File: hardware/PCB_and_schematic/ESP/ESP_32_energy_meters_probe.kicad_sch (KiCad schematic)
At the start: 31 parts, among them J2 Conn_01x10, J5 METER_GRID, J9 METER_PV, U4 ST485EBDR, U5 ST485EBDR, U6 74HC14

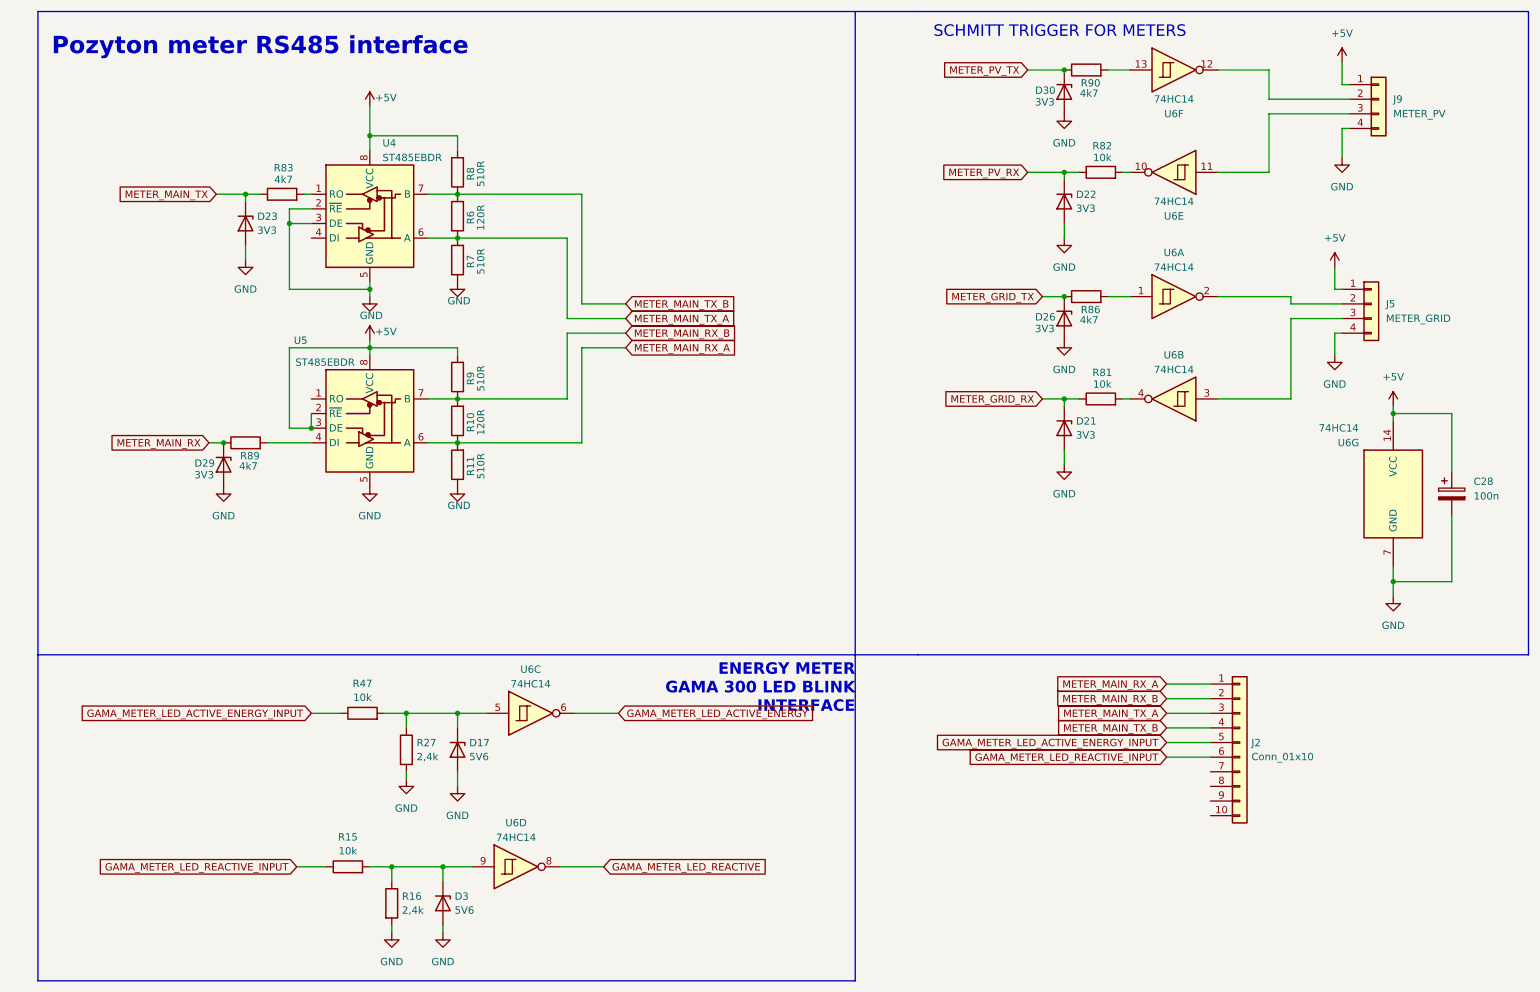
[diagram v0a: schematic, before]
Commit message: Routing PCB
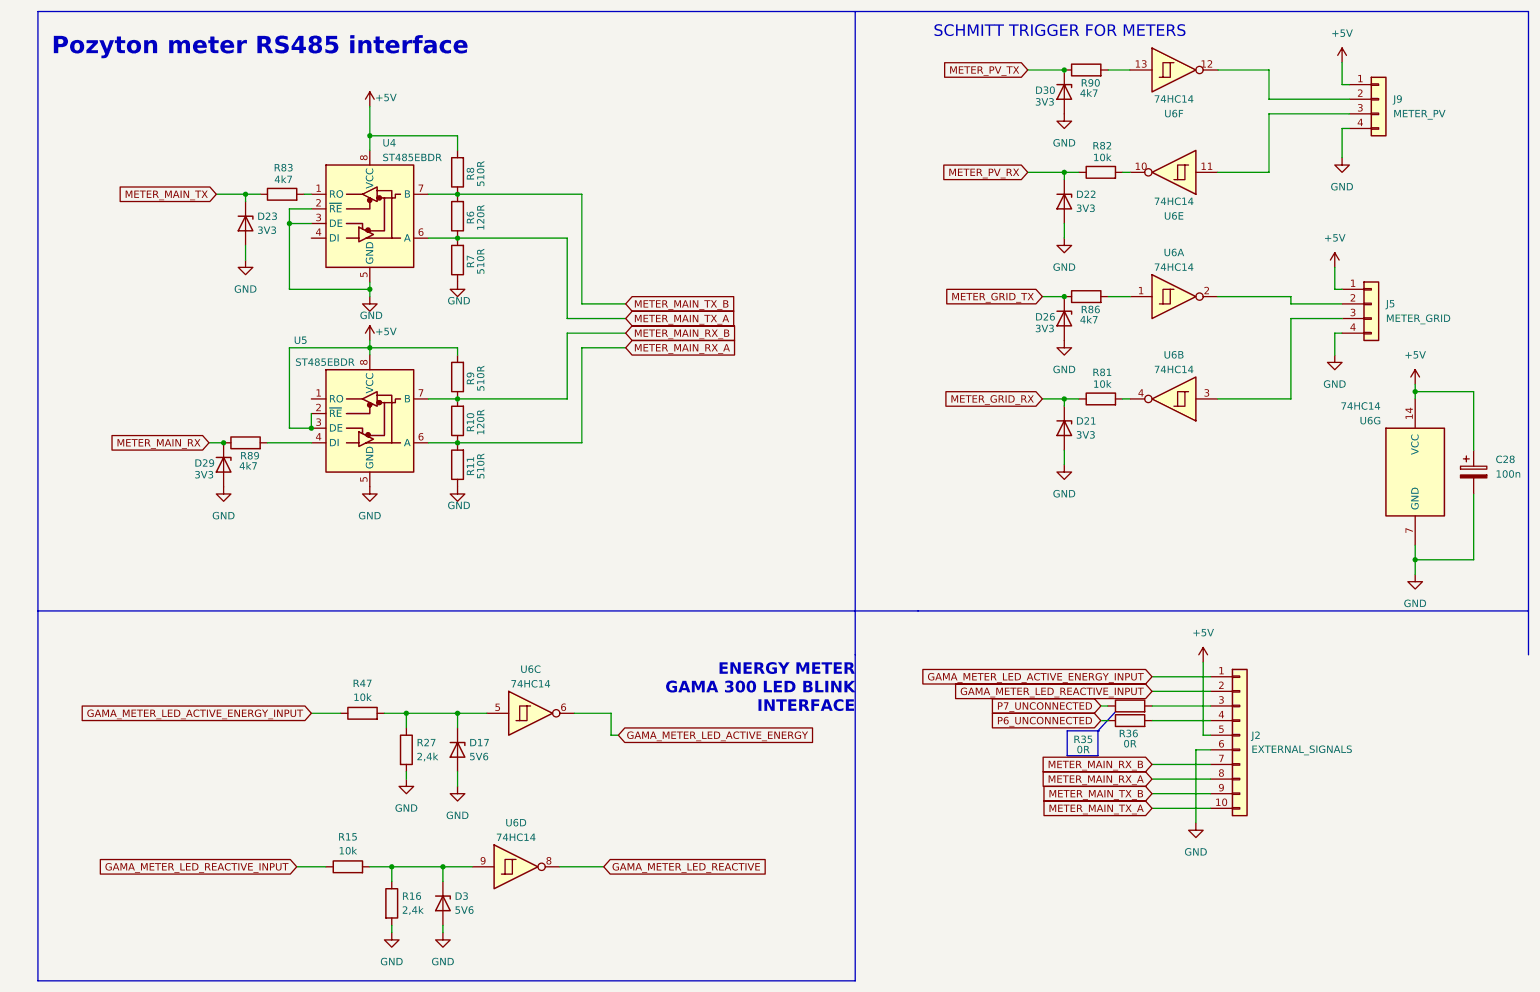
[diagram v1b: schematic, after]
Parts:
- added R35, R36: 0R, Resistor_SMD:R_0805_2012Metric_Pad1.20x1.40mm_HandSolder, symbol Device:R
- J2: value Conn_01x10 -> EXTERNAL_SIGNALS
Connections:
- net +5V: now also J2.5 (Pin_5)
- net GAMA_METER_LED_ACTIVE_ENERGY_INPUT: now also J2.1 (Pin_1); no longer J2.5 (Pin_5)
- net GAMA_METER_LED_REACTIVE_INPUT: now also J2.2 (Pin_2); no longer J2.6 (Pin_6)
- net GND: now also J2.6 (Pin_6)
- net METER_MAIN_RX_A: now also J2.8 (Pin_8); no longer J2.1 (Pin_1)
- net METER_MAIN_RX_B: now also J2.7 (Pin_7); no longer J2.2 (Pin_2)
- net METER_MAIN_TX_A: now also J2.10 (Pin_10); no longer J2.3 (Pin_3)
- net METER_MAIN_TX_B: now also J2.9 (Pin_9); no longer J2.4 (Pin_4)
- new net: J2.3 (Pin_3), R35.2
- new net: J2.4 (Pin_4), R36.2
- new net P6_UNCONNECTED: R36.1
- new net P7_UNCONNECTED: R35.1
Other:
- moved on the sheet: C28, J2, U6G
